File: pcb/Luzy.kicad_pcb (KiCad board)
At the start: 2 copper layers, 33 x 50.8 mm, 64 parts, among them J1 Battery Connector, P1 USB_C_Plug_USB2.0, SW1 POWER/MODE, SW2 LEFT, SW3 RIGHT, SW4 RESET, U1 TLV61070A, U2 LM3671, U3 ESP32-C3, U4 SN74LVC1T45DBV, U5 BQ25170JDSGR, Y1 32.768kHz 12.5pF, Y2 40MHz 12pF

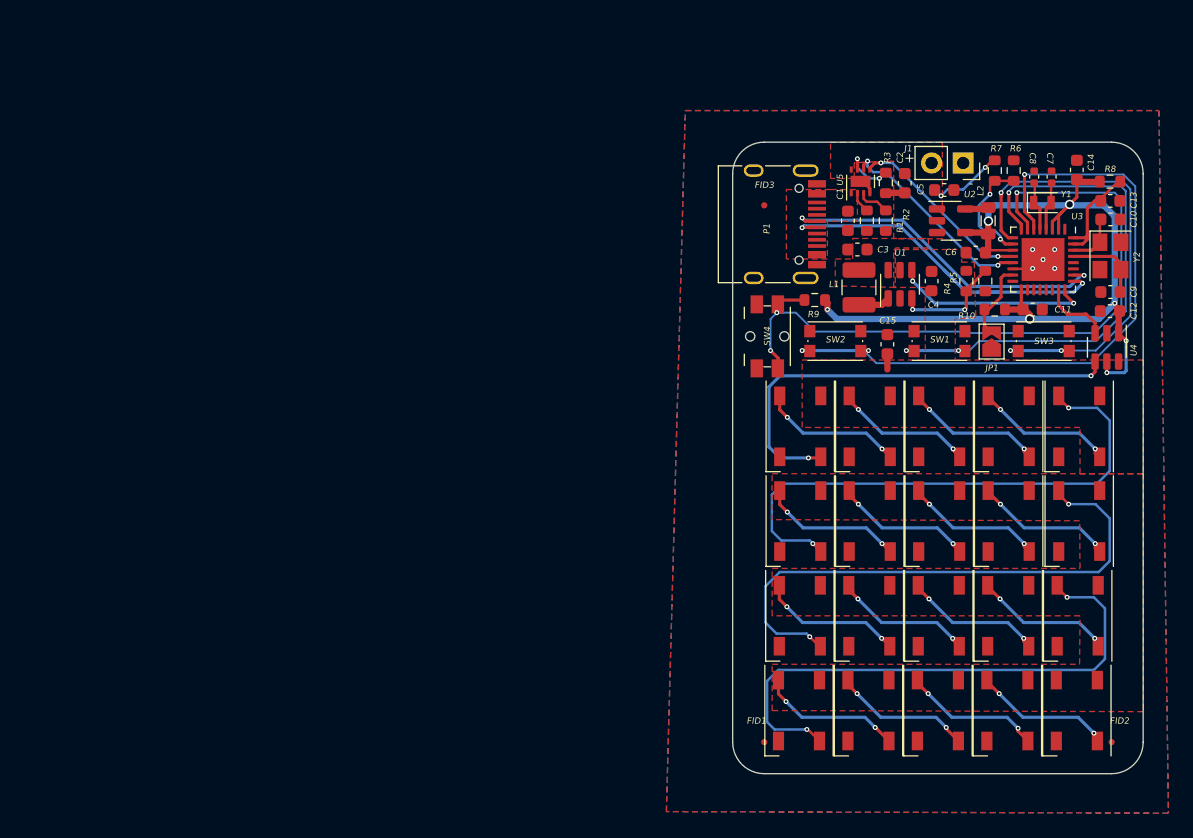
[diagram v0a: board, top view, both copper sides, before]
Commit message: Finished First Version
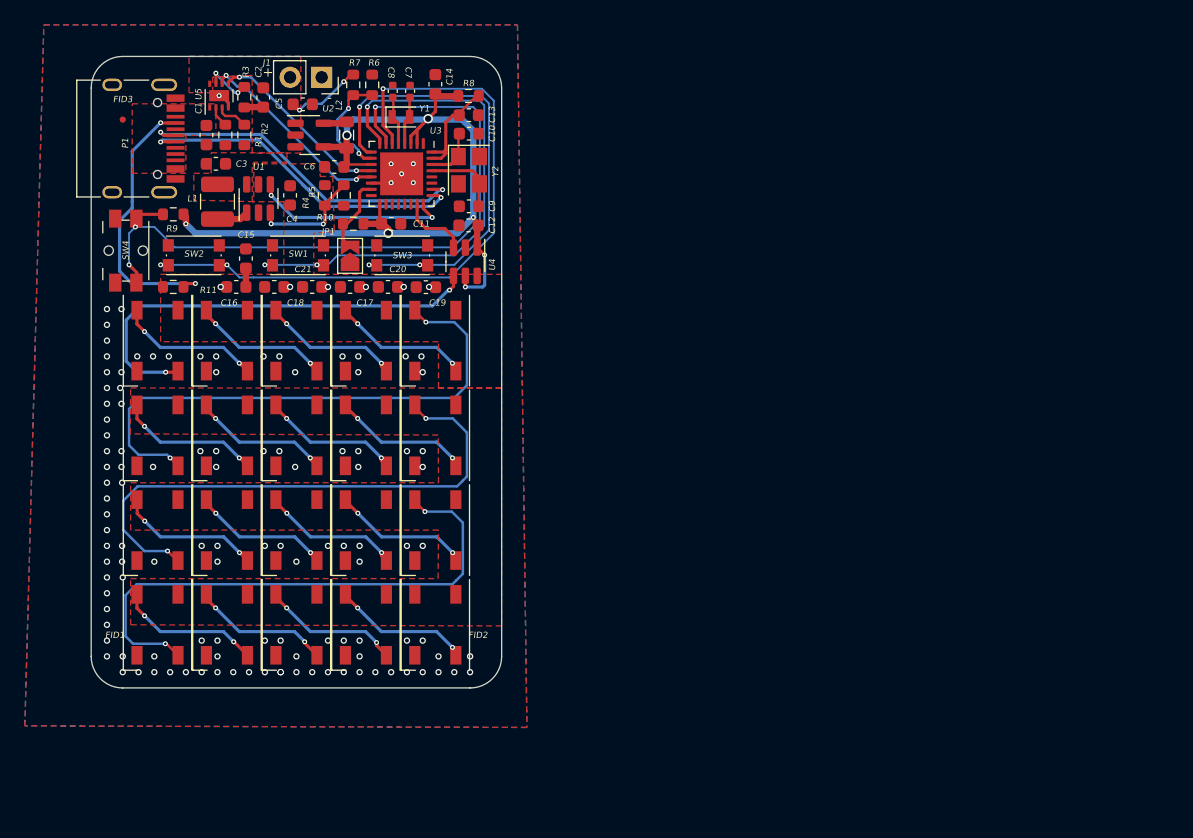
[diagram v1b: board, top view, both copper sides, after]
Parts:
- added C16: 4.7uF, Capacitor_SMD:C_0603_1608Metric, F.Cu at (93.4, 57.4)
- added C17: 4.7uF, Capacitor_SMD:C_0603_1608Metric, F.Cu at (102.6, 57.4)
- added C18: 4.7uF, Capacitor_SMD:C_0603_1608Metric, F.Cu at (96.5, 57.4)
- added C19: 4.7uF, Capacitor_SMD:C_0603_1608Metric, F.Cu at (108.7, 57.4)
- added C20: 4.7uF, Capacitor_SMD:C_0603_1608Metric, F.Cu at (105.6, 57.4)
- added C21: 4.7uF, Capacitor_SMD:C_0603_1608Metric, F.Cu at (99.5, 57.4)
- added G***: LOGO, LOGO, B.Cu at (98.9, 65.3)
- added R11: 5.1k, Resistor_SMD:R_0603_1608Metric, F.Cu at (88.4, 57.4)
- P1: value USB_C_Plug_USB2.0 -> USB4105
- SW1: value POWER/MODE -> KMR211
- SW2: value LEFT -> KMR211
- SW3: value RIGHT -> KMR211
- SW4: value RESET -> EVQ-PUM02K
- moved D10 52.3 mm to (109.4, 69.3)
- moved D5 52.3 mm to (109.4, 61.7)
- moved D4 52.2 mm to (103.8, 61.7)
- moved D9 52.2 mm to (103.8, 69.3)
- moved D1 52.2 mm to (87.1, 61.7)
- moved D2 52.2 mm to (92.7, 61.7)
- moved D6 52.2 mm to (87.1, 69.3)
- moved D7 52.2 mm to (92.7, 69.3)
- moved D3 52.2 mm to (98.3, 61.7)
- moved D8 52.2 mm to (98.3, 69.3)
- moved D13 52.1 mm to (98.3, 76.9)
- moved D14 52.1 mm to (103.8, 76.9)
- moved D15 52.1 mm to (109.4, 76.9)
- moved D11 52.1 mm to (87.1, 76.9)
- moved D12 52.1 mm to (92.7, 76.9)
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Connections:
- P1 pad A5: unconnected-(P1-PadA5) -> Net-(P1-PadA5)
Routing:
- net Net-(P1-PadA5): track 0.00 -> 22.1 mm, vias 0 -> 2
- net /DATA: track 36.8 -> 35.9 mm
- net /GND: track 4.25 -> 4.30 mm, vias 5 -> 126
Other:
- board text added: "Version 1.0a Orion Serup"
